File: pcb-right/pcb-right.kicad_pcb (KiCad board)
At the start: 2 copper layers, 124.8 x 104.5 mm, 43 parts, among them J2 BAT, U2 xiao-ble

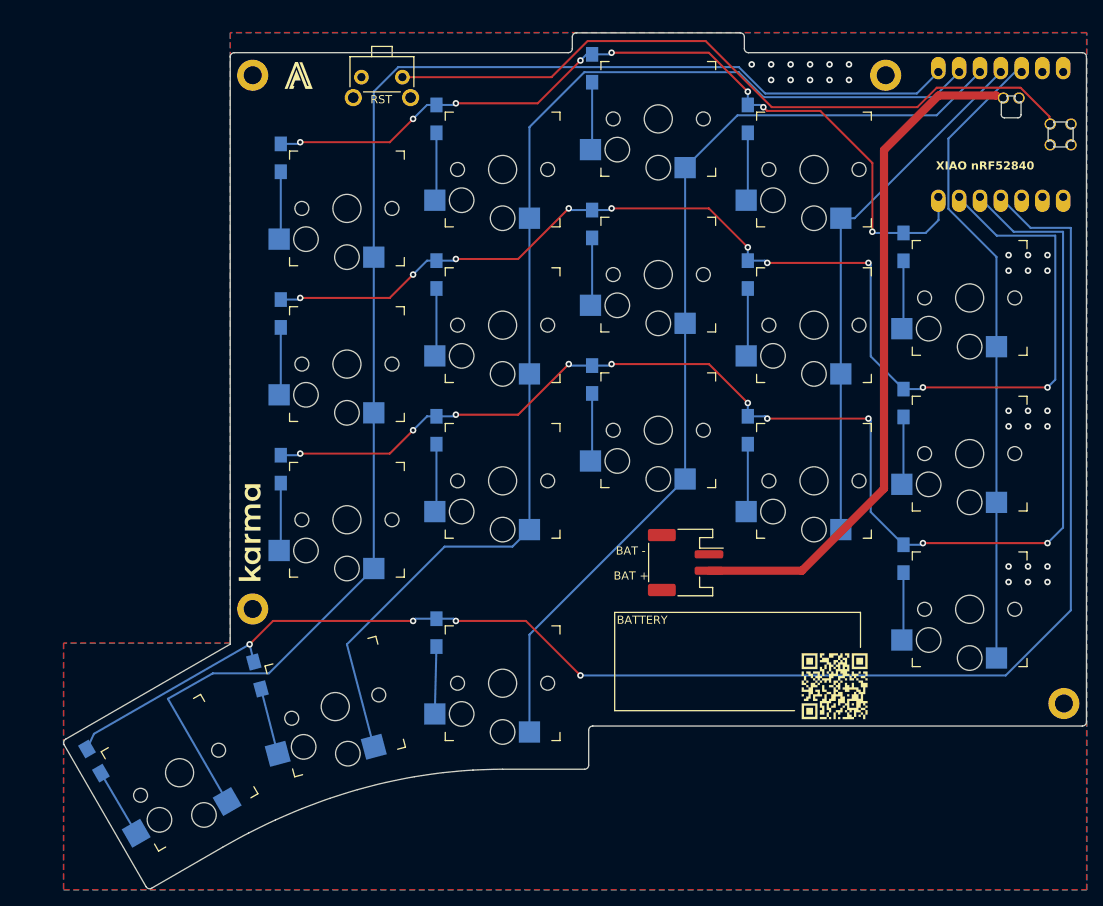
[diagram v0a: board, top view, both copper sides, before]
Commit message: Right Positioned
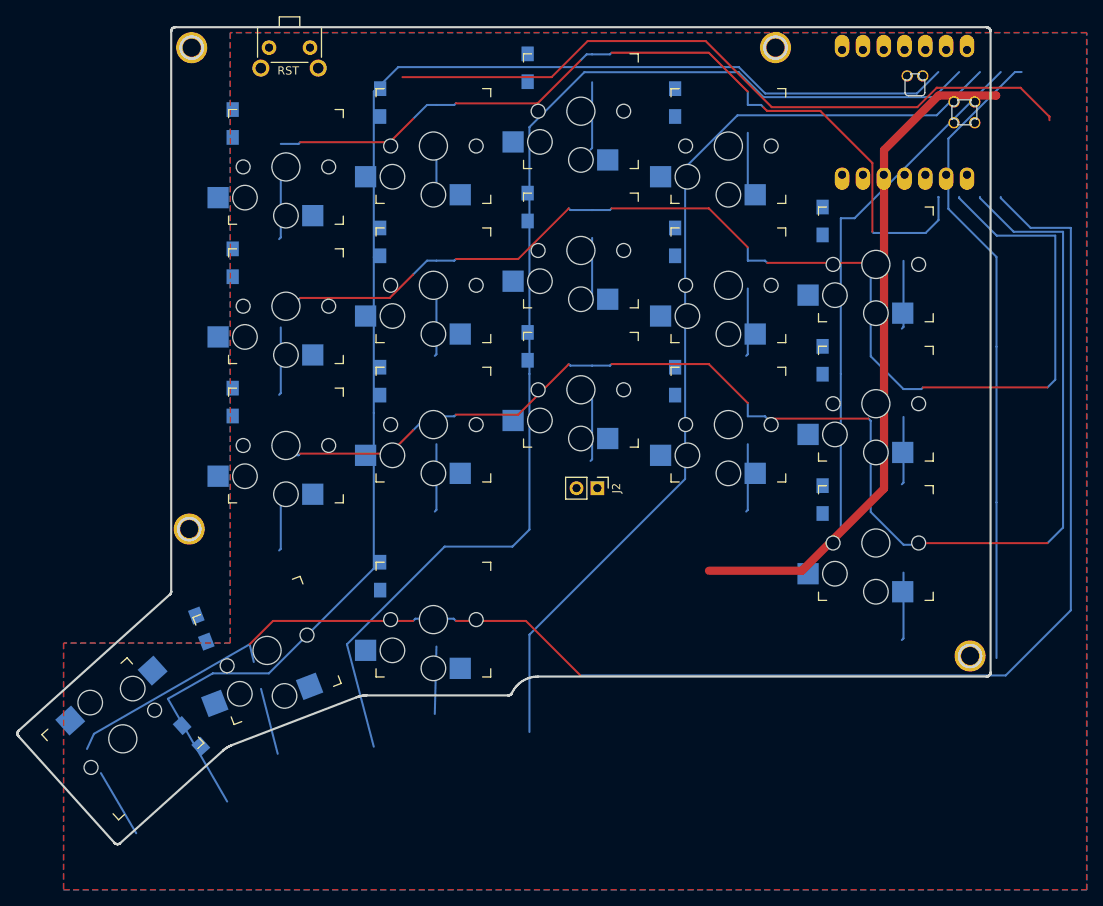
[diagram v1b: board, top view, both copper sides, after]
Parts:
- J2: footprint Connector_JST:JST_PH_S2B-PH-SM4-TB_1x02-1MP_P2.00mm_Horizontal -> Connector_PinHeader_2.54mm:PinHeader_1x02_P2.54mm_Vertical
- moved SWR15 26.3 mm to (127.0, 84.5)
- moved SWR10 25.1 mm to (127.0, 67.5)
- moved SWR14 24.8 mm to (109.0, 70.0)
- moved SWR11 24.1 mm to (55.0, 72.5)
- moved SWR5 24.0 mm to (127.0, 50.5)
- moved SWR9 23.6 mm to (109.0, 53.0)
- moved SWR12 23.2 mm to (73.0, 70.0)
- moved SWR13 22.8 mm to (91.0, 65.8)
- moved SWR6 22.6 mm to (55.0, 55.5)
- moved SWR4 22.5 mm to (109.0, 36.0)
- moved SWR7 22.0 mm to (73.0, 53.0)
- moved SWR8 21.7 mm to (91.0, 48.8)
- moved SWR1 21.3 mm to (55.0, 38.5)
- moved SWR2 20.8 mm to (73.0, 36.0)
- moved SWR3 20.7 mm to (91.0, 31.8)
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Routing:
- net Net-(DR2-A): track 8.31 -> 184.8 mm
- net COL4_R: track 176.5 -> 0.00 mm
- net Net-(DR5-A): track 8.36 -> 170.8 mm
- net Net-(DR11-A): track 8.31 -> 156.2 mm
- net COL3_R: track 147.9 -> 0.00 mm
- net ROW3_R: track 190.7 -> 44.5 mm, vias 4 -> 0
- net GND_R: track 0.00 -> 78.1 mm, vias 29 -> 0
- net ROW2_R: track 165.8 -> 95.4 mm, vias 10 -> 0
- net ROW1_R: track 147.7 -> 115.0 mm, vias 10 -> 0
- net Net-(DR1-A): track 8.78 -> 35.0 mm
- net COL1_R: track 64.9 -> 89.8 mm
- net COL0_R: track 78.1 -> 57.7 mm
- net Net-(DR15-A): track 8.31 -> 19.6 mm
- net Net-(DR4-A): track 8.31 -> 0.00 mm
- net Net-(DR9-A): track 8.31 -> 0.00 mm
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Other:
- board size 124.8 x 104.5 mm -> 118.8 x 99.7 mm
- board text removed: "BAT +"
- board text removed: "BAT -"
- board text removed: "BATTERY"
- board text removed: "XIAO nRF52840"
